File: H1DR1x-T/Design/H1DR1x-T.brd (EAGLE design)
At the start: 34.6 x 30 mm, 30 parts, among them P1 HEXABIT_17.32_NO_P6, P2 RS-485, U1 STM32G0B1CEU6QFN_B1CEU6_STM-L, U2 MAX14840EASAT, X1 XTALL_CSTCE8M00G52

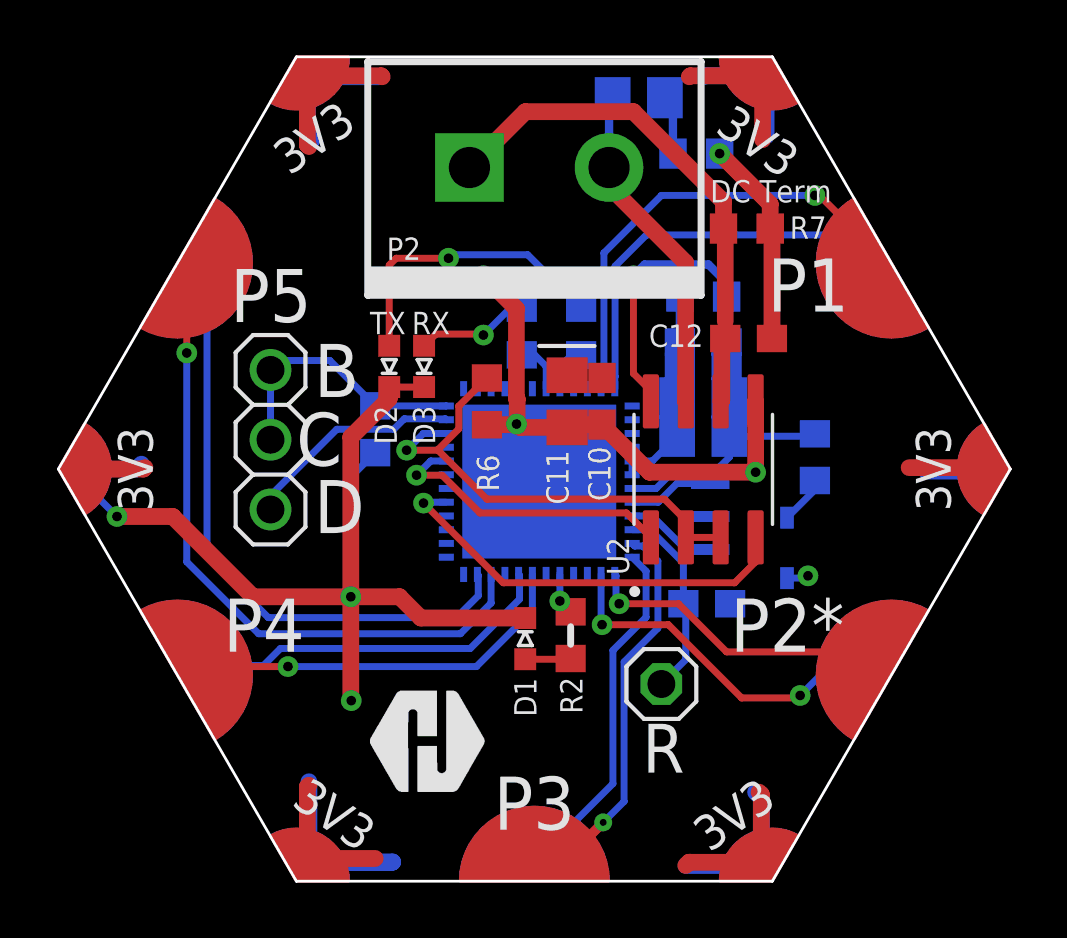
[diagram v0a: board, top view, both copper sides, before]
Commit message: Everything is finished. I fixed some issues and reviewed everything.
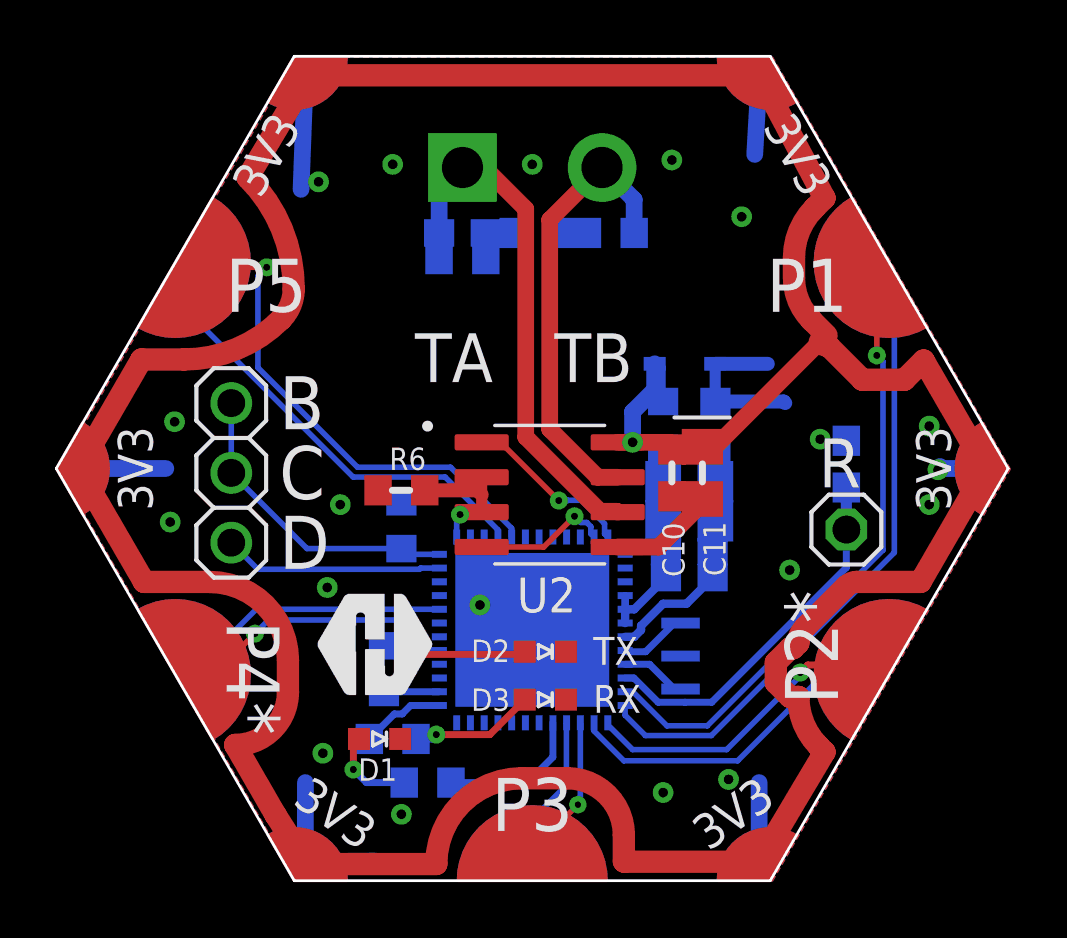
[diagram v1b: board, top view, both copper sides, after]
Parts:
- removed C1: 1uF, HEXABITZ_RCLS:C-0805
- added C2: 1uF, HEXABITZ_RCLS:C-0805
- C10, C12: device Hexabitz:C-0603 -> HEXABITZ_RCLS:C-0603
- C11: device Hexabitz:C-0805-POL -> HEXABITZ_RCLS:C-0805-POL
- P2: device Hexabitz:1546111-2 -> HEXABITZ_CONNECTION_PARTS:1546111-2
- R1: value 0.0R -> 270R
- R2: value 270R -> 0.0R
- R4, R6, R7: device Hexabitz:R-0603 -> HEXABITZ_RCLS:R-0603
- R5: device Hexabitz:R-0805 -> HEXABITZ_RCLS:R-0603
- R8, R9: value 270.0R -> 270R
- U2: value MAX14840EASAT -> MAX14840EASA+T; device Hexabitz:SOIC127P600X175-8N -> HEXABITZ_ICs:SOIC127P600X175-8N
- moved R1 18.4 mm to (-3.81, 3.65), turned to 0 degrees
- moved R9 15.6 mm to (-5.08, 5.24), turned to 0 degrees
- moved R8 14.2 mm to (-5.40, 7.78)
- moved D3 12.9 mm to (0.48, 6.67), turned to 90 degrees
- moved D2 11.8 mm to (0.48, 8.41), turned to 90 degrees
- moved C12 11.1 mm to (-2.54, 23.7), flipped to the bottom, turned to 180 degrees
- moved R7 10.4 mm to (-2.54, 22.7), flipped to the bottom, turned to 0 degrees
- moved R2 9.29 mm to (6.67, 16.7), flipped to the bottom
- moved R 8.77 mm to (11.4, 12.9)
- moved C5 7.70 mm to (5.71, 11.1)
- moved D5 7.66 mm to (5.56, 18.9), turned to 0 degrees
- moved C6 7.64 mm to (5.71, 12.1)
- moved C3 7.18 mm to (11.4, 15.2), turned to 90 degrees
- moved R4 6.49 mm to (0.16, 23.7), turned to 0 degrees
- moved D1 6.44 mm to (-5.56, 5.24), turned to 90 degrees
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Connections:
- net N$7 renamed TB
- net N$8 renamed TA
- removed net N$11: R9.2, U1.43
- removed net N$9: R8.2, U1.44
- removed net UART1_RTS: R6.1, U1.34, U2.2, U2.3
- removed net UART1_RX: U1.32, U2.1
- removed net UART1_TX: U1.29, U2.4
- new net RX_LED: R9.2, U1.25
- new net TX_LED: R8.2, U1.26
- new net USART1_RX: P1.PAD_PD4, U1.32
- new net USART1_TX: P1.PAD_PU4, U1.29
- new net USART3_RTS: R6.1, U1.37, U2.2, U2.3
- net GND: now also R2.1; no longer R1.1
- net N$1: now also R1.2; no longer R2.2
- net N$3: now also R1.1; no longer R2.1
- net USART3_RX: now also U1.48, U2.1; no longer P1.PAD_PD5, U1.23
- net USART3_TX: now also U1.47, U2.4; no longer P1.PAD_PU5, U1.22
- net USART4_RX: now also P1.PAD_PD1; no longer P1.PAD_PD3
- net USART4_TX: now also P1.PAD_PU1; no longer P1.PAD_PU3
- net USART5_RX: now also P1.PAD_PD5, U1.40; no longer P1.PAD_PD4, U1.20
- net USART5_TX: now also P1.PAD_PU5, U1.41; no longer P1.PAD_PU4, U1.19
- net USART6_RX: now also P1.PAD_PD3, U1.16; no longer P1.PAD_PD1, U1.48
- net USART6_TX: now also P1.PAD_PU3, U1.15; no longer P1.PAD_PU1, U1.47
- net VDDA: now also C2.1; no longer C1.1
- net VSSA: now also C2.2, R2.2; no longer C1.2, R1.2
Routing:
- net VDD: track 36.6 -> 130.8 mm, vias 2 -> 1
- net GND: track 87.8 -> 50.3 mm, vias 6 -> 19
- net USART3_TX: track 24.3 -> 5.02 mm
- net UART1_RTS: track 18.2 -> 0.00 mm, vias 1 -> 0
- net USART3_RX: track 23.7 -> 6.24 mm, vias 0 -> 1
- net UART1_TX: track 15.3 -> 0.00 mm, vias 1 -> 0
- net USART6_TX: track 17.3 -> 5.78 mm
- net UART1_RX: track 10.8 -> 0.00 mm, vias 1 -> 0
- net USART4_RX: track 13.0 -> 23.8 mm
- net USART1_TX: track 0.00 -> 10.1 mm, vias 0 -> 1
- net USART1_RX: track 0.00 -> 9.85 mm
- net USART6_RX: track 15.0 -> 5.57 mm
- net USART4_TX: track 14.8 -> 22.8 mm
- net N$4: track 7.19 -> 13.4 mm
- net N$13: track 10.9 -> 5.29 mm
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- added copper zone on layer 1, net GND
- removed copper zone on layer 1, net VDD
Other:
- board text added: "*"
- board text added: "P4*"
- board text removed: "P4"
